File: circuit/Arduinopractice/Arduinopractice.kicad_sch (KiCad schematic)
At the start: 0 parts

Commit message: いろいろ追加
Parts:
- added C2: 0.1u, Capacitor_SMD:C_0603_1608Metric_Pad1.08x0.95mm_HandSolder, symbol Device:C
- added D1, D2, D3: LED, LED_SMD:LED_0805_2012Metric, symbol Device:LED
- added IC1: MB1010-000, Meister:MB1010000, symbol Meister:MB1010-000
- added J1: XIAORP2040, RF_Module:MCU_Seeed_ESP32C3, symbol Connector:Conn_01x14_Pin
- added Q1: 2SC1815, Package_TO_SOT_THT:TO-92_Inline, symbol Transistor_BJT:2SC1815
- added R1, R2, R3: 330, Resistor_SMD:R_0805_2012Metric, symbol Device:R
- added R4: 1k, Resistor_SMD:R_0603_1608Metric_Pad0.98x0.95mm_HandSolder, symbol Device:R
- added R5, R6: 10k, Resistor_SMD:R_0603_1608Metric_Pad0.98x0.95mm_HandSolder, symbol Device:R
- added R7: 10k, Resistor_SMD:R_0805_2012Metric, symbol Device:R
- added R8, R9: 4.7k, Resistor_SMD:R_0805_2012Metric, symbol Device:R
- added SHT31: Conn_01x05_Socket, Connector_PinHeader_2.54mm:PinHeader_1x05_P2.54mm_Vertical, symbol Connector:Conn_01x05_Socket
- added SW1: SW_Push_Dual, Button_Switch_THT:SW_PUSH_6mm_H4.3mm, symbol Switch:SW_Push_Dual
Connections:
- new net: D2.2 (A), R2.2
- new net: J1.1 (Pin_1), R1.1
- new net: D1.2 (A), R1.2
- new net: IC1.5 (TX), R5.2, R6.2
- new net: J1.2 (Pin_2), R2.1
- new net: D3.2 (A), R3.2
- new net: J1.3 (Pin_3), R3.1
- new net: Q1.3 (B), R5.1
- new net +3V3: C2.1, IC1.6 (+5), J1.12 (Pin_12), R4.2, R7.2, R8.2, R9.1, SHT31.1 (Pin_1)
- new net Analog: IC1.3 (AN), J1.4 (Pin_4)
- new net GND: C2.2, IC1.1 (BW), IC1.7 (GND), J1.13 (Pin_13), Q1.1 (E), R6.1, SHT31.5 (Pin_5), SW1.4
- new net PWM: IC1.2 (PW), J1.9 (Pin_9)
- new net RX: J1.8 (Pin_8), Q1.2 (C), R4.1
- new net SCL: J1.6 (Pin_6), R8.1, SHT31.3 (Pin_3)
- new net SDA: J1.5 (Pin_5), R9.2, SHT31.2 (Pin_2)
- new net SW: J1.10 (Pin_10), R7.1, SW1.1
- no-connect marks 0 -> 9
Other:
- note added: "疑似RS232なのでNOT回路を挟む。"

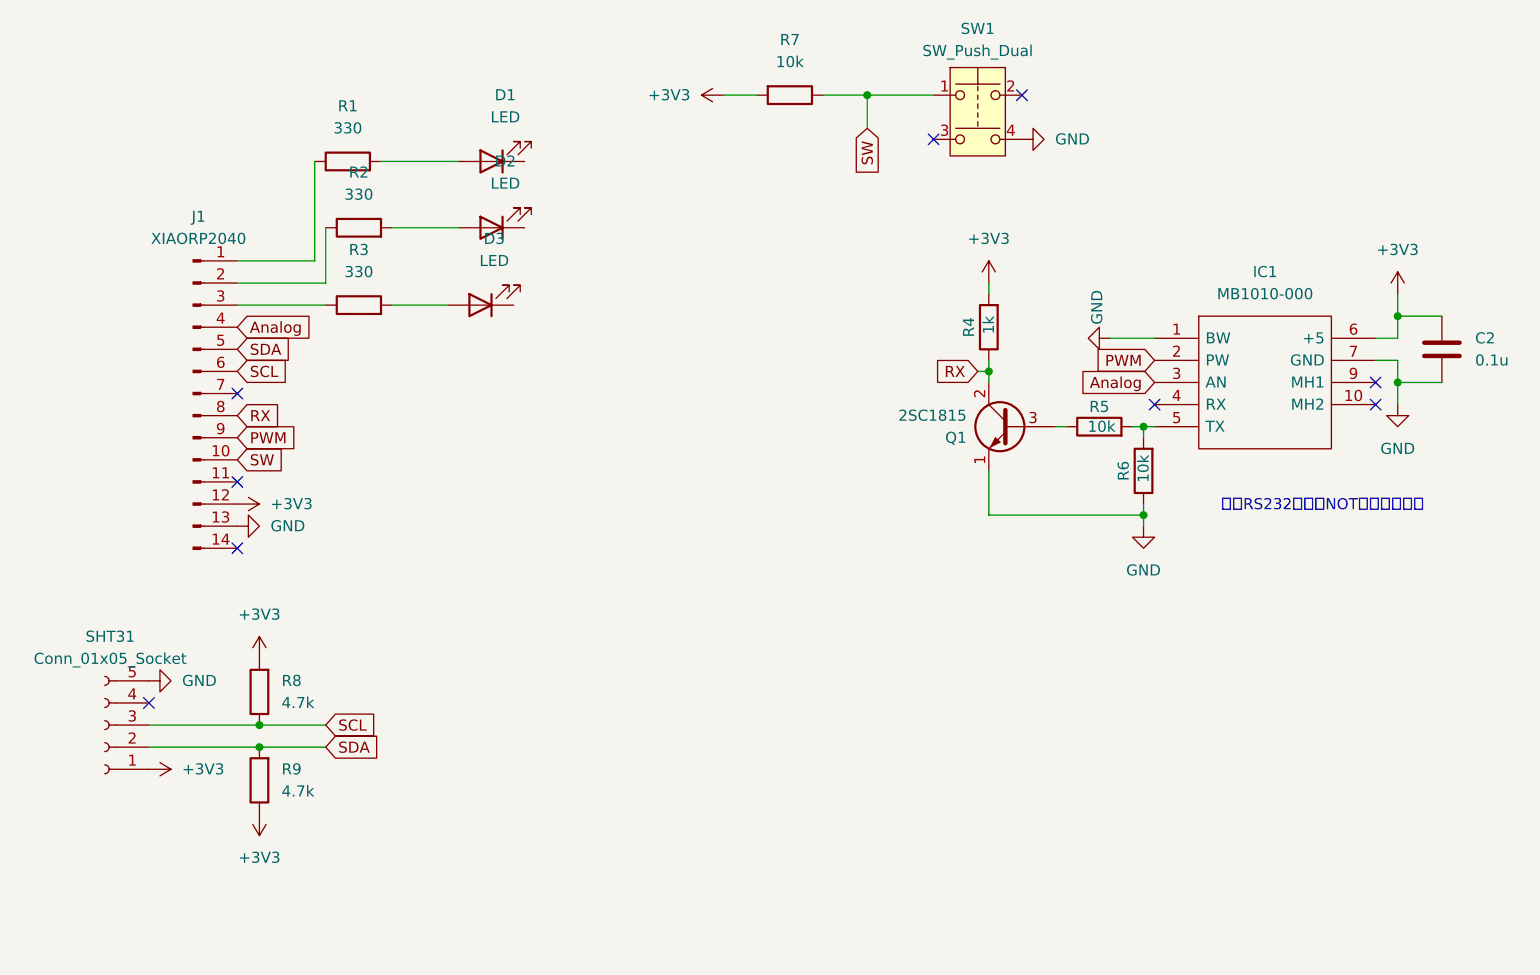
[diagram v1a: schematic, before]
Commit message: シンボルを変更
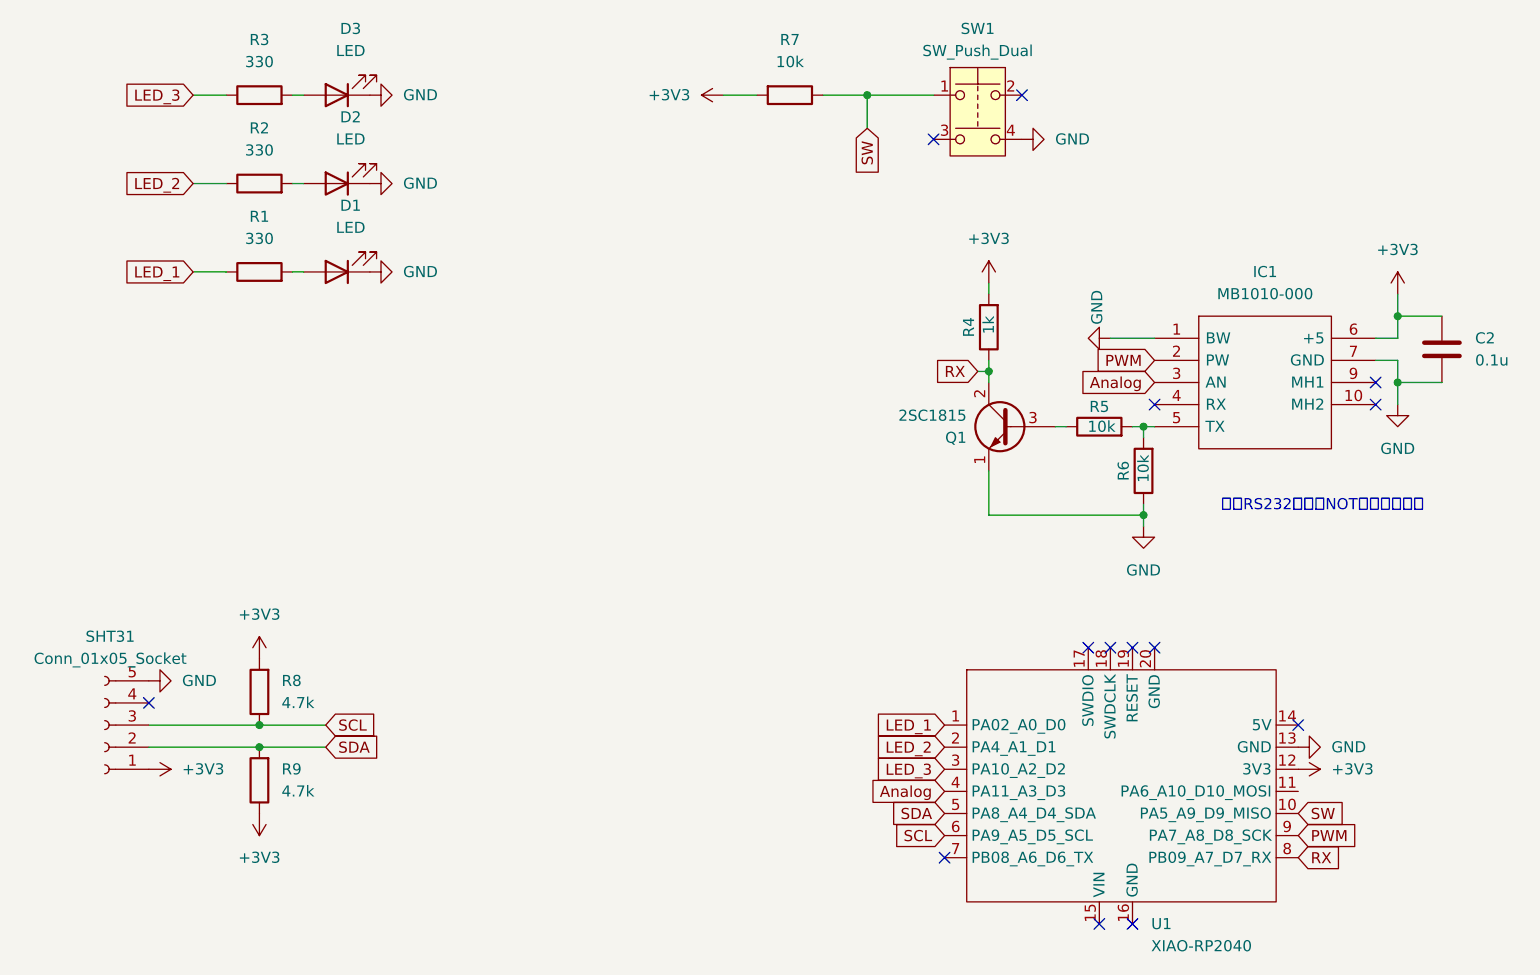
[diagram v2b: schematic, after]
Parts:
- removed J1: XIAORP2040, RF_Module:MCU_Seeed_ESP32C3, symbol Connector:Conn_01x14_Pin
- added U1: XIAO-RP2040, Meister:Seeeduino XIAO-MOUDLE14P-2.54-21X17.8MM, symbol Meister:MOUDLE-SEEEDUINO-XIAO
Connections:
- net +3V3: now also U1.12 (3V3)
- net Analog: now also U1.4 (PA11_A3_D3)
- net GND: now also D1.1 (K), D2.1 (K), D3.1 (K), U1.13 (GND)
- net PWM: now also U1.9 (PA7_A8_D8_SCK)
- net RX: now also U1.8 (PB09_A7_D7_RX)
- net SCL: now also U1.6 (PA9_A5_D5_SCL)
- net SDA: now also U1.5 (PA8_A4_D4_SDA)
- net SW: now also U1.10 (PA5_A9_D9_MISO)
- net LED_1: now reaches R1.1
- net LED_1: now also U1.1 (PA02_A0_D0)
- net LED_2: now reaches R2.1
- net LED_2: now also U1.2 (PA4_A1_D1)
- net LED_3: now reaches R3.1
- net LED_3: now also U1.3 (PA10_A2_D2)
- no-connect marks 9 -> 14
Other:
- moved on the sheet: D2, D3, R2, R3
